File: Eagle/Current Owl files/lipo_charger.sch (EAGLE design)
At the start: 23 parts, among them J1 2X6 FEMALE, J2 2X6 FEMALE, Q1 2N3906, X1 SMA-142-0701-851/861

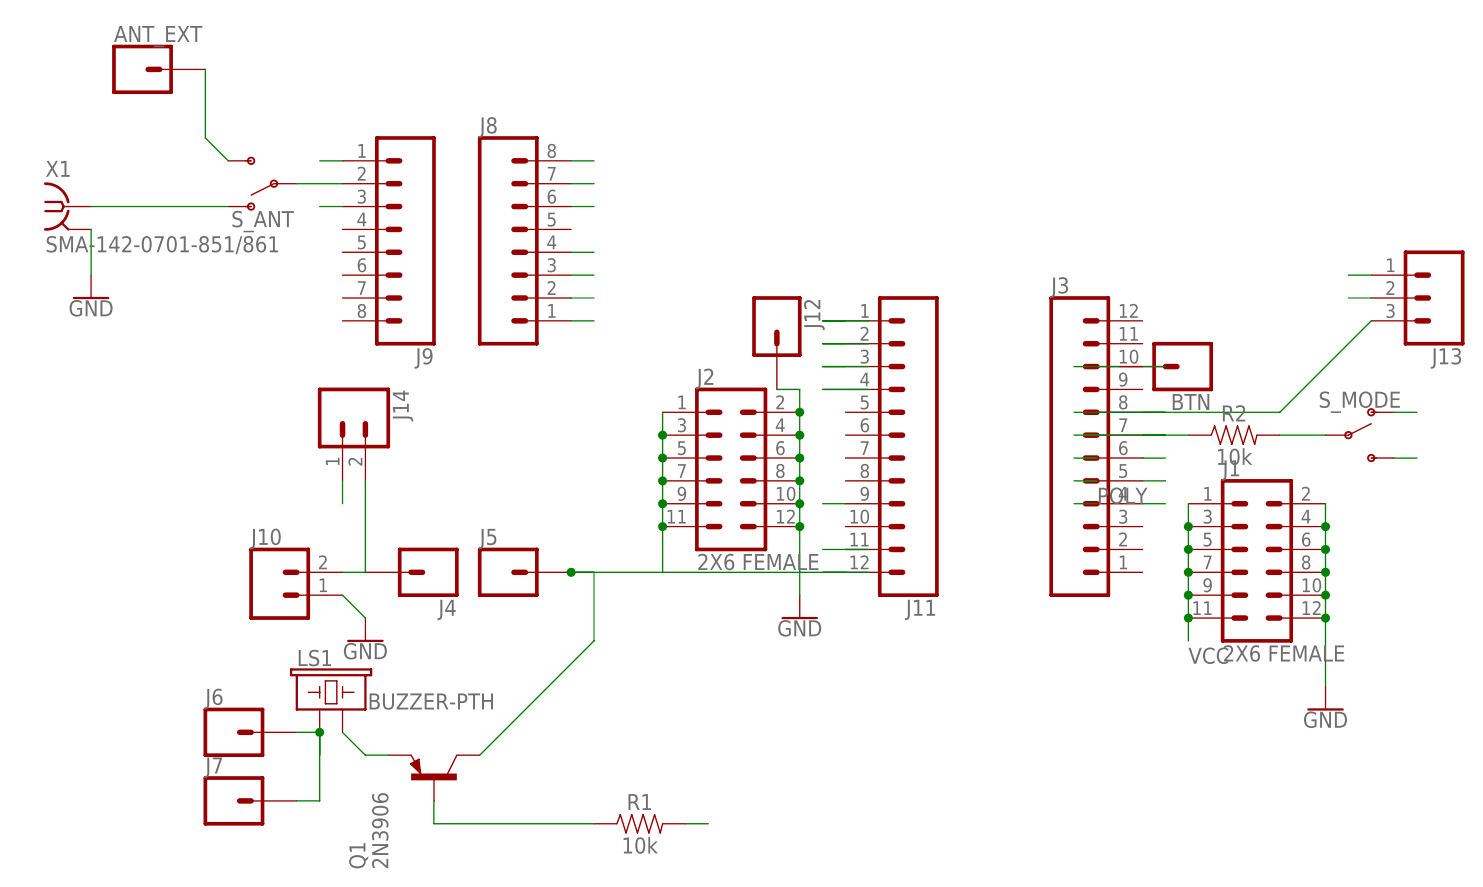
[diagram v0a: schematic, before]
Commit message: updated eagle files
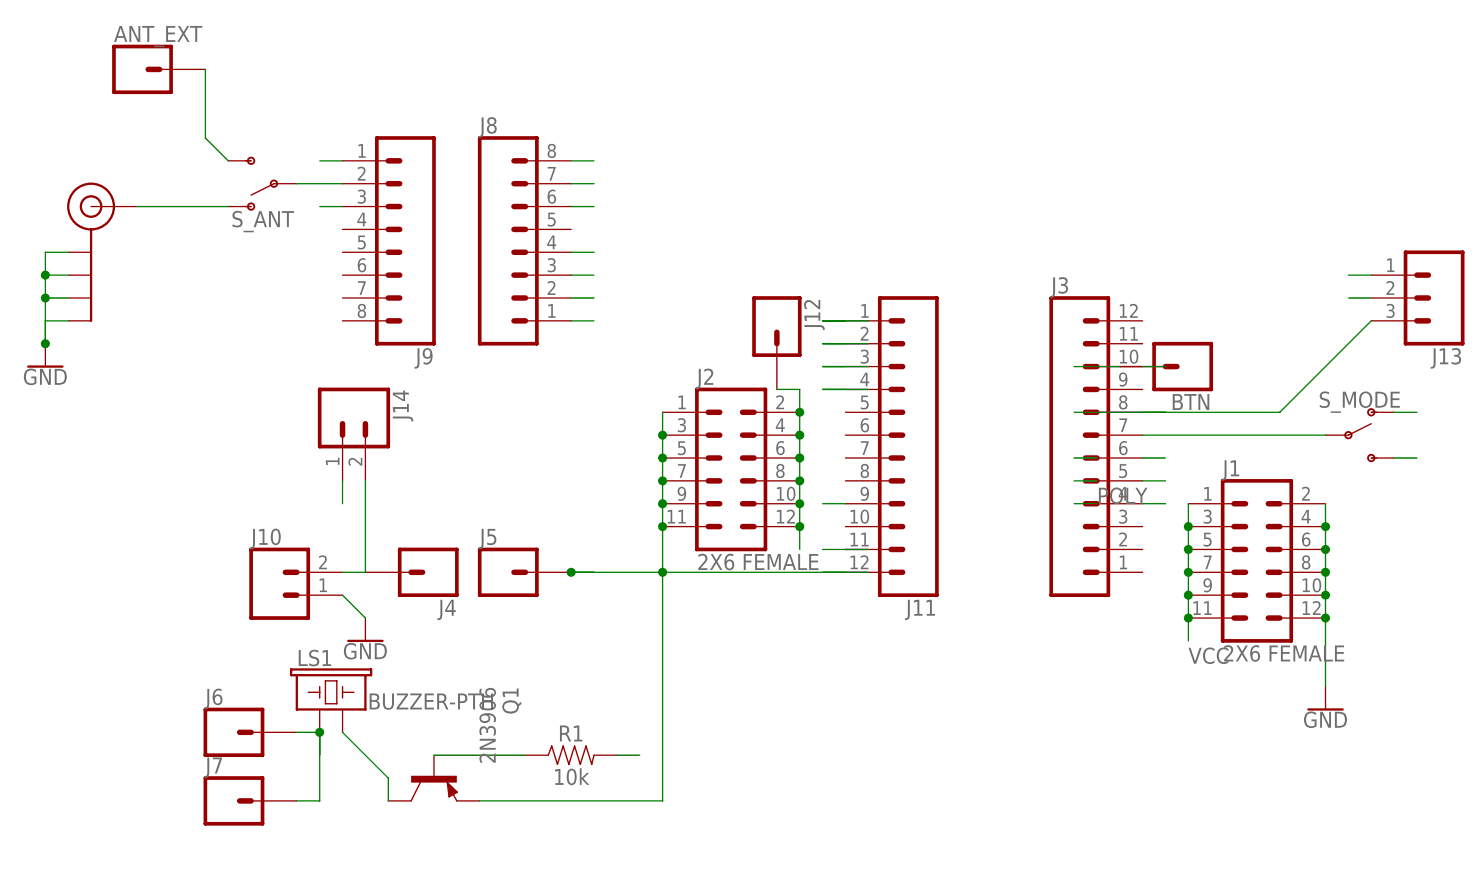
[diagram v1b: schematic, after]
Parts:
- removed R2: 10k, SparkFun-Resistors:10KOHM-HORIZ-1/6W-5%
- removed X1: SMA-142-0701-851/861, con-coax:SMA-142-0701-851/861
- added J$1: SMA_EDGE, SparkFun-Retired:SMA_EDGE
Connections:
- removed net 7: J3.7, R2.1
- net GND: now also J$1.GND@0, J$1.GND@1, J$1.GND@2, J$1.GND@3; no longer X1.2
- net N$3: now also Q1.C; no longer Q1.E
- net N$6: now also J3.7; no longer R2.2
- net N$8: now also J$1.SIGNAL; no longer X1.1
- net RAW: now also Q1.E; no longer Q1.C
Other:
- moved on the sheet: Q1, R1
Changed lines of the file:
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@@
 <part name="J2" library="SparkFun-Connectors" deviceset="CONN_06X2" device="PTH_FEMALE" value="2X6 FEMALE"/>
 <part name="S_MODE" library="SparkFun-Switches" deviceset="SWITCH-SPDT" device="-PTH-11.6X4.0MM"/>
-<part name="X1" library="con-coax" deviceset="SMA-" device="142-0701-851/861"/>
 <part name="LS1" library="SparkFun-Electromechanical" deviceset="BUZZER" device="-PTH"/>
 <part name="Q1" library="transistor-pnp" deviceset="2N3906" device=""/>
@@
 <part name="ANT_EXT" library="SparkFun-Connectors" deviceset="CONN_01" device=""/>
 <part name="GND1" library="SparkFun-PowerSymbols" deviceset="GND" device=""/>
-<part name="GND2" library="SparkFun-PowerSymbols" deviceset="GND" device=""/>
 <part name="GND3" library="SparkFun-PowerSymbols" deviceset="GND" device=""/>
 <part name="GND5" library="SparkFun-PowerSymbols" deviceset="GND" device=""/>
@@
 <part name="J13" library="SparkFun-Connectors" deviceset="CONN_03" device="JST-PTH"/>
 <part name="J14" library="SparkFun-Connectors" deviceset="CONN_02" device=""/>
-<part name="R2" library="SparkFun-Resistors" deviceset="10KOHM" device="-HORIZ-1/6W-5%" value="10k"/>
+<part name="J$1" library="SparkFun-Retired" deviceset="SMA_EDGE" device=""/>
 </parts>
 <sheets>
@@
 <instance part="J2" gate="G$1" x="114.3" y="93.98"/>
 <instance part="S_MODE" gate="1" x="185.42" y="104.14"/>
-<instance part="X1" gate="G1" x="43.18" y="129.54"/>
 <instance part="LS1" gate="G$1" x="71.12" y="73.66"/>
-<instance part="Q1" gate="G$1" x="83.82" y="66.04" rot="R90"/>
+<instance part="Q1" gate="G$1" x="83.82" y="66.04" rot="R270"/>
 <instance part="S_ANT" gate="1" x="66.04" y="132.08" rot="R180"/>
 <instance part="ANT_EXT" gate="G$1" x="50.8" y="144.78"/>
 <instance part="GND1" gate="1" x="182.88" y="73.66"/>
-<instance part="GND2" gate="1" x="124.46" y="83.82"/>
-<instance part="GND3" gate="1" x="45.72" y="119.38"/>
+<instance part="GND3" gate="1" x="40.64" y="111.76"/>
 <instance part="GND5" gate="1" x="76.2" y="81.28"/>
 <instance part="BTN" gate="G$1" x="167.64" y="111.76" rot="R180"/>
 <instance part="J4" gate="G$1" x="83.82" y="88.9" rot="R180"/>
 <instance part="J5" gate="G$1" x="91.44" y="88.9"/>
-<instance part="R1" gate="G$1" x="106.68" y="60.96"/>
+<instance part="R1" gate="G$1" x="99.06" y="68.58"/>
 <instance part="J6" gate="G$1" x="60.96" y="71.12"/>
 <instance part="J7" gate="G$1" x="60.96" y="63.5"/>
@@
 <instance part="J13" gate="J$1" x="195.58" y="119.38" rot="R180"/>
 <instance part="J14" gate="G$1" x="73.66" y="106.68" rot="R270"/>
-<instance part="R2" gate="G$1" x="172.72" y="104.14"/>
+<instance part="J$1" gate="1" x="45.72" y="129.54"/>
 </instances>
 <busses>
@@
 <wire x1="109.22" y1="93.98" x2="109.22" y2="88.9" width="0.1524" layer="91"/>
 <wire x1="132.08" y1="88.9" x2="109.22" y2="88.9" width="0.1524" layer="91"/>
-<pinref part="Q1" gate="G$1" pin="C"/>
-<wire x1="88.9" y1="68.58" x2="101.6" y2="81.28" width="0.1524" layer="91"/>
-<wire x1="101.6" y1="81.28" x2="101.6" y2="88.9" width="0.1524" layer="91"/>
 <pinref part="J5" gate="G$1" pin="1"/>
 <junction x="99.06" y="88.9"/>
+<pinref part="Q1" gate="G$1" pin="E"/>
+<wire x1="88.9" y1="63.5" x2="109.22" y2="63.5" width="0.1524" layer="91"/>
+<wire x1="109.22" y1="63.5" x2="109.22" y2="88.9" width="0.1524" layer="91"/>
+<junction x="109.22" y="88.9"/>
 </segment>
 <segment>
@@
 </segment>
 </net>
-<net name="7" class="0">
-<segment>
-<pinref part="R2" gate="G$1" pin="1"/>
-<wire x1="167.64" y1="104.14" x2="154.94" y2="104.14" width="0.1524" layer="91"/>
-</segment>
-<segment>
-<pinref part="J3" gate="G$1" pin="7"/>
-<wire x1="162.56" y1="104.14" x2="165.1" y2="104.14" width="0.1524" layer="91"/>
-</segment>
-</net>
 <net name="N$3" class="0">
 <segment>
 <pinref part="LS1" gate="G$1" pin="2"/>
-<pinref part="Q1" gate="G$1" pin="E"/>
-<wire x1="73.66" y1="71.12" x2="76.2" y2="68.58" width="0.1524" layer="91"/>
-<wire x1="76.2" y1="68.58" x2="78.74" y2="68.58" width="0.1524" layer="91"/>
+<pinref part="Q1" gate="G$1" pin="C"/>
+<wire x1="78.74" y1="63.5" x2="78.74" y2="66.04" width="0.1524" layer="91"/>
+<wire x1="78.74" y1="66.04" x2="73.66" y2="71.12" width="0.1524" layer="91"/>
 </segment>
 </net>
 <net name="SPKR" class="0">
 <segment>
-<wire x1="111.76" y1="60.96" x2="114.3" y2="60.96" width="0.1524" layer="91"/>
+<wire x1="104.14" y1="68.58" x2="106.68" y2="68.58" width="0.1524" layer="91"/>
 <pinref part="R1" gate="G$1" pin="2"/>
 </segment>
@@
 <wire x1="68.58" y1="132.08" x2="73.66" y2="132.08" width="0.1524" layer="91"/>
 <pinref part="J9" gate="G$1" pin="2"/>
-</segment>
-</net>
-<net name="N$8" class="0">
-<segment>
-<pinref part="S_ANT" gate="1" pin="O"/>
-<pinref part="X1" gate="G1" pin="1"/>
-<wire x1="60.96" y1="129.54" x2="45.72" y2="129.54" width="0.1524" layer="91"/>
 </segment>
 </net>
@@
 </segment>
 <segment>
-<pinref part="X1" gate="G1" pin="2"/>
-<wire x1="45.72" y1="127" x2="45.72" y2="121.92" width="0.1524" layer="91"/>
-<pinref part="GND3" gate="1" pin="GND"/>
-</segment>
-<segment>
 <pinref part="GND5" gate="1" pin="GND"/>
 <wire x1="76.2" y1="83.82" x2="73.66" y2="86.36" width="0.1524" layer="91"/>
 <pinref part="J10" gate="G$1" pin="1"/>
-</segment>
-<segment>
-<pinref part="J2" gate="G$1" pin="2"/>
-<pinref part="J2" gate="G$1" pin="4"/>
-<wire x1="124.46" y1="106.68" x2="124.46" y2="104.14" width="0.1524" layer="91"/>
-<pinref part="J2" gate="G$1" pin="6"/>
-<wire x1="124.46" y1="101.6" x2="124.46" y2="104.14" width="0.1524" layer="91"/>
-<junction x="124.46" y="104.14"/>
-<pinref part="J2" gate="G$1" pin="8"/>
-<wire x1="124.46" y1="101.6" x2="124.46" y2="99.06" width="0.1524" layer="91"/>
-<junction x="124.46" y="101.6"/>
-<pinref part="J2" gate="G$1" pin="10"/>
-<wire x1="124.46" y1="99.06" x2="124.46" y2="96.52" width="0.1524" layer="91"/>
-<junction x="124.46" y="99.06"/>
-<pinref part="J2" gate="G$1" pin="12"/>
-<wire x1="124.46" y1="96.52" x2="124.46" y2="93.98" width="0.1524" layer="91"/>
-<junction x="124.46" y="96.52"/>
-<pinref part="GND2" gate="1" pin="GND"/>
-<wire x1="124.46" y1="93.98" x2="124.46" y2="86.36" width="0.1524" layer="91"/>
-<junction x="124.46" y="93.98"/>
-<pinref part="J12" gate="G$1" pin="1"/>
-<wire x1="121.92" y1="109.22" x2="124.46" y2="109.22" width="0.1524" layer="91"/>
-<wire x1="124.46" y1="109.22" x2="124.46" y2="106.68" width="0.1524" layer="91"/>
-<junction x="124.46" y="106.68"/>
 </segment>
 <segment>
@@
 <wire x1="73.66" y1="99.06" x2="73.66" y2="96.52" width="0.1524" layer="91"/>
 </segment>
+<segment>
+<pinref part="J2" gate="G$1" pin="2"/>
+<pinref part="J2" gate="G$1" pin="4"/>
+<wire x1="124.46" y1="106.68" x2="124.46" y2="104.14" width="0.1524" layer="91"/>
+<pinref part="J2" gate="G$1" pin="6"/>
+<wire x1="124.46" y1="101.6" x2="124.46" y2="104.14" width="0.1524" layer="91"/>
+<junction x="124.46" y="104.14"/>
+<pinref part="J2" gate="G$1" pin="8"/>
+<wire x1="124.46" y1="101.6" x2="124.46" y2="99.06" width="0.1524" layer="91"/>
+<junction x="124.46" y="101.6"/>
+<pinref part="J2" gate="G$1" pin="10"/>
+<wire x1="124.46" y1="99.06" x2="124.46" y2="96.52" width="0.1524" layer="91"/>
+<junction x="124.46" y="99.06"/>
+<pinref part="J2" gate="G$1" pin="12"/>
+<wire x1="124.46" y1="96.52" x2="124.46" y2="93.98" width="0.1524" layer="91"/>
+<junction x="124.46" y="96.52"/>
+<pinref part="J12" gate="G$1" pin="1"/>
+<wire x1="121.92" y1="109.22" x2="124.46" y2="109.22" width="0.1524" layer="91"/>
+<wire x1="124.46" y1="109.22" x2="124.46" y2="106.68" width="0.1524" layer="91"/>
+<junction x="124.46" y="106.68"/>
+<wire x1="124.46" y1="93.98" x2="124.46" y2="91.44" width="0.1524" layer="91"/>
+<junction x="124.46" y="93.98"/>
+</segment>
+<segment>
+<pinref part="J$1" gate="1" pin="GND@0"/>
+<pinref part="GND3" gate="1" pin="GND"/>
+<wire x1="43.18" y1="124.46" x2="40.64" y2="124.46" width="0.1524" layer="91"/>
+<wire x1="40.64" y1="124.46" x2="40.64" y2="121.92" width="0.1524" layer="91"/>
+<pinref part="J$1" gate="1" pin="GND@1"/>
+<wire x1="40.64" y1="121.92" x2="40.64" y2="119.38" width="0.1524" layer="91"/>
+<wire x1="40.64" y1="119.38" x2="40.64" y2="114.3" width="0.1524" layer="91"/>
+<wire x1="43.18" y1="121.92" x2="40.64" y2="121.92" width="0.1524" layer="91"/>
+<junction x="40.64" y="121.92"/>
+<pinref part="J$1" gate="1" pin="GND@2"/>
+<wire x1="43.18" y1="119.38" x2="40.64" y2="119.38" width="0.1524" layer="91"/>
+<junction x="40.64" y="119.38"/>
+<pinref part="J$1" gate="1" pin="GND@3"/>
+<wire x1="43.18" y1="116.84" x2="40.64" y2="116.84" width="0.1524" layer="91"/>
+<wire x1="40.64" y1="116.84" x2="40.64" y2="114.3" width="0.1524" layer="91"/>
+<junction x="40.64" y="114.3"/>
+</segment>
+</net>
+<net name="N$9" class="0">
+<segment>
+<pinref part="J14" gate="G$1" pin="2"/>
+<wire x1="76.2" y1="99.06" x2="76.2" y2="88.9" width="0.1524" layer="91"/>
+</segment>
 </net>
 <net name="N$1" class="0">
@@
 <pinref part="R1" gate="G$1" pin="1"/>
 <pinref part="Q1" gate="G$1" pin="B"/>
-<wire x1="101.6" y1="60.96" x2="83.82" y2="60.96" width="0.1524" layer="91"/>
-<wire x1="83.82" y1="60.96" x2="83.82" y2="63.5" width="0.1524" layer="91"/>
-</segment>
-</net>
-<net name="N$9" class="0">
-<segment>
-<pinref part="J14" gate="G$1" pin="2"/>
-<wire x1="76.2" y1="99.06" x2="76.2" y2="88.9" width="0.1524" layer="91"/>
+<wire x1="93.98" y1="68.58" x2="83.82" y2="68.58" width="0.1524" layer="91"/>
 </segment>
 </net>
 <net name="N$6" class="0">
 <segment>
+<pinref part="J3" gate="G$1" pin="7"/>
 <pinref part="S_MODE" gate="1" pin="P"/>
-<wire x1="182.88" y1="104.14" x2="177.8" y2="104.14" width="0.1524" layer="91"/>
-<pinref part="R2" gate="G$1" pin="2"/>
-</segment>
-</net>
+<wire x1="162.56" y1="104.14" x2="182.88" y2="104.14" width="0.1524" layer="91"/>
+</segment>
+</net>
+<net name="N$8" class="0">
+<segment>
+<pinref part="J$1" gate="1" pin="SIGNAL"/>
+<pinref part="S_ANT" gate="1" pin="O"/>
+<wire x1="50.8" y1="129.54" x2="60.96" y2="129.54" width="0.1524" layer="91"/>
+</segment>
+</net>
